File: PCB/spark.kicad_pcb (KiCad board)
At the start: 2 copper layers, 145.2 x 137.5 mm, 38 parts, among them SW1 SW_Push_45deg, SW10 SW_Push_45deg, SW11 SW_Push_45deg, SW12 SW_Push_45deg, SW13 SW_Push_45deg, SW14 SW_Push_45deg, SW15 SW_Push_45deg, SW16 SW_Push_45deg, SW17 SW_Push_45deg, SW18 SW_Push_45deg, SW2 SW_Push_45deg, SW20 Reset Switch, SW3 SW_Push_45deg, SW4 SW_Push_45deg, SW5 SW_Push_45deg, SW6 SW_Push_45deg, SW7 SW_Push_45deg, SW8 SW_Push_45deg, SW9 SW_Push_45deg, U1 SuperMini nRF52840

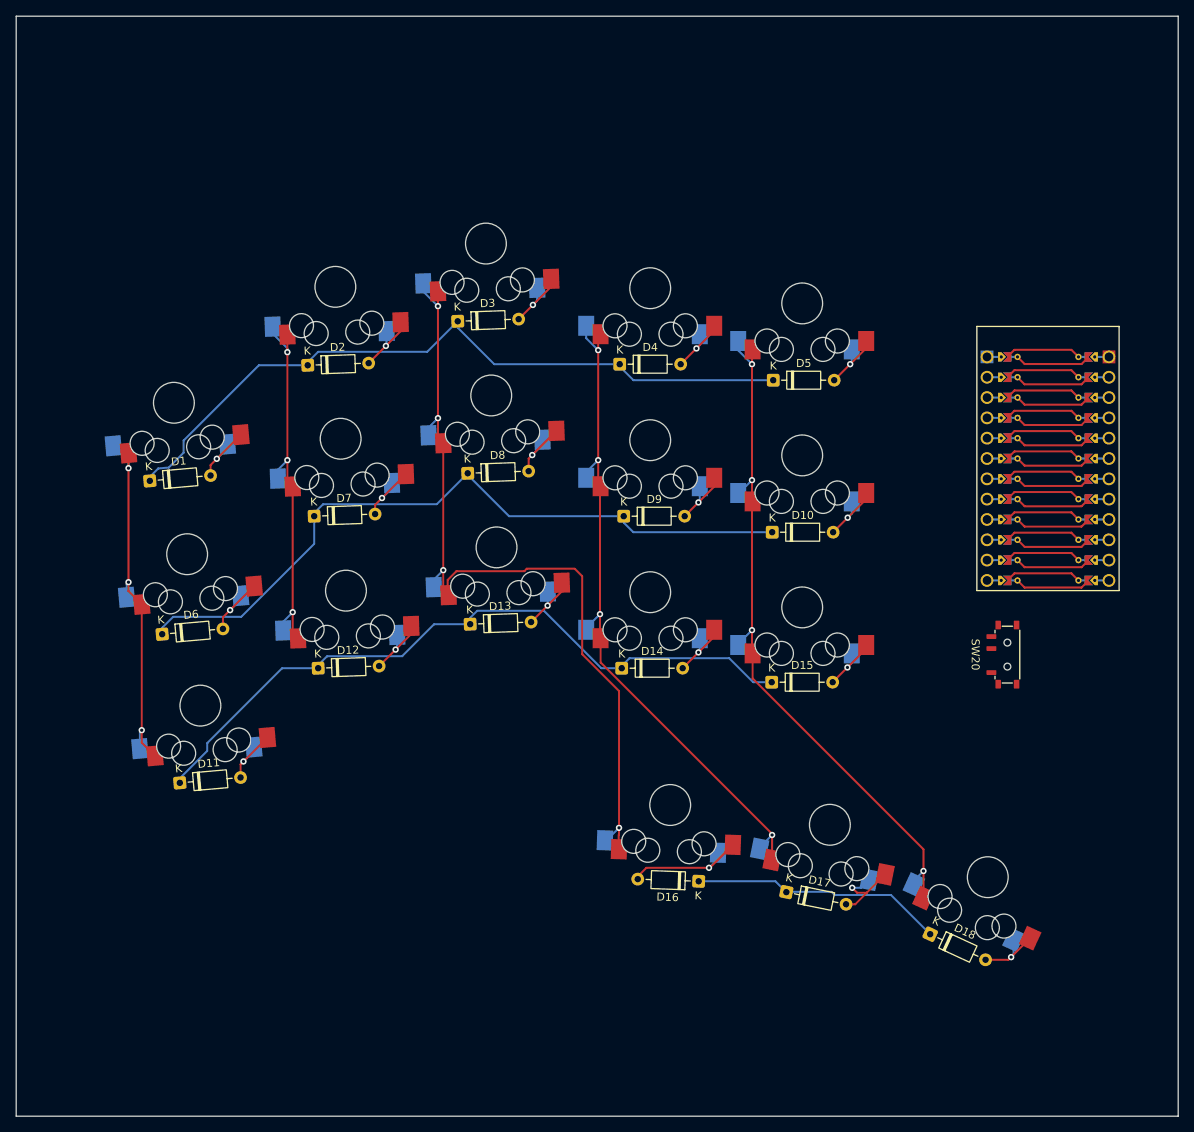
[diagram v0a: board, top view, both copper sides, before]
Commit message: Routed everything
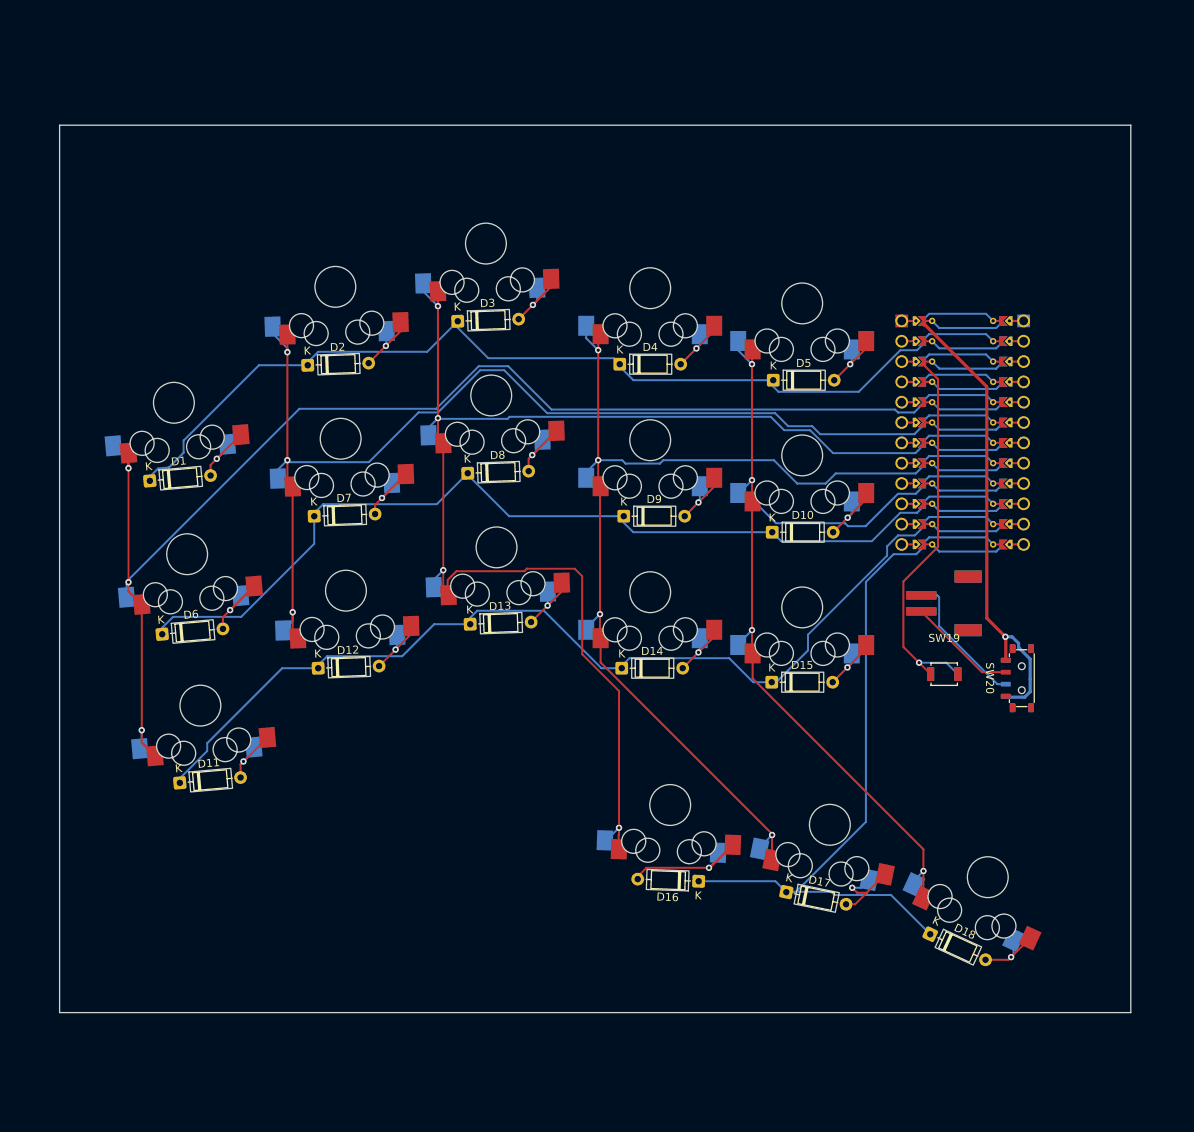
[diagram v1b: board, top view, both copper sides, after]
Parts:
- added J1: JST connector, KiCAD_Stuff:Connector_1x02_JST-PH, F.Cu at (167.1, 132.1)
- added SW19: Reset Switch, KiCAD_Stuff:SW_SPST_B3U-1000P_Reversible, F.Cu at (167.0, 141.0)
- D1, D10, D11, D12, D13, D14, D15, D16, D17, D18, D2, D3, D4, D5, D6, D7, D8, D9: footprint Diode_THT:D_DO-35_SOD27_P7.62mm_Horizontal -> KiCAD_Stuff:1N4148 Cutout Diode
- SW20: value Reset Switch -> Power Switch; footprint PCM_marbastlib-various:SW_MSK12C02-HB -> PCM_marbastlib-various:SW_MSK12C02-HB_Reversible
- U1: value SuperMini nRF52840 -> Nice_Nano_V2
- moved U1 8.94 mm to (169.3, 110.8)
- moved SW20 3.46 mm to (176.7, 141.5)
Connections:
- SW20 pad 2: unconnected-(SW20A-B-Pad2) -> JST_Bat+
- SW20 pad 3: unconnected-(SW20A-C-Pad3) -> Bat+
- U1 pad 10: Row1 -> Row2
- U1 pad 11: Row2 -> Row3
- U1 pad 12: Row3 -> Row4
- U1 pad 2: unconnected-(U1-P0.08-Pad2) -> Row1
- U1 pad 22: unconnected-(U1-P1.11-LF-Pad22) -> Reset
- U1 pad 23: unconnected-(U1-P0.10-LF-Pad23) -> GND
- U1 pad 24: Row4 -> Bat+
- U1 pad 3: unconnected-(U1-GND-Pad3) -> GND
- U1 pad 4: unconnected-(U1-GND-Pad4) -> GND
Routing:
- net Col1: track 47.2 -> 160.8 mm
- net Col2: track 48.0 -> 136.3 mm
- net Col3: track 105.6 -> 168.2 mm
- net Bat+: track 0.00 -> 58.2 mm, vias 0 -> 1
- net Row4: track 31.7 -> 84.4 mm
- net Reset: track 0.00 -> 48.3 mm, vias 0 -> 1
- net Col4: track 86.4 -> 129.7 mm
- net JST_Bat+: track 0.00 -> 31.0 mm
- net Row3: track 89.4 -> 118.3 mm
- net Col5: track 88.3 -> 115.7 mm
- net Row1: track 91.2 -> 113.7 mm
- net Row2: track 90.9 -> 112.2 mm
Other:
- board size 145.2 x 137.5 mm -> 133.9 x 110.9 mm
